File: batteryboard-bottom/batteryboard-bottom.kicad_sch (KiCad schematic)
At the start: 6 parts, among them J1 SLM-110-01-G-S, J2 FTS-105-01-L-DV-A

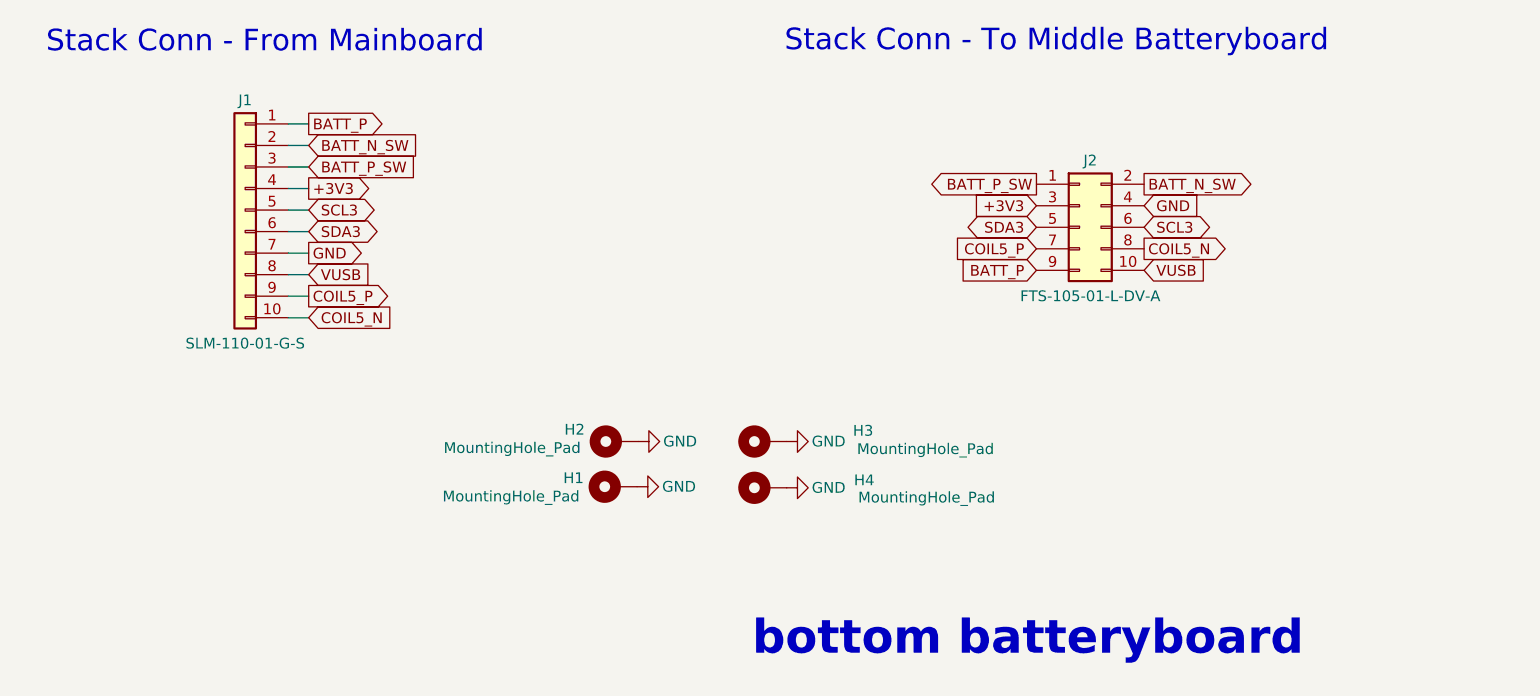
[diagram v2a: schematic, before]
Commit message: Some changes
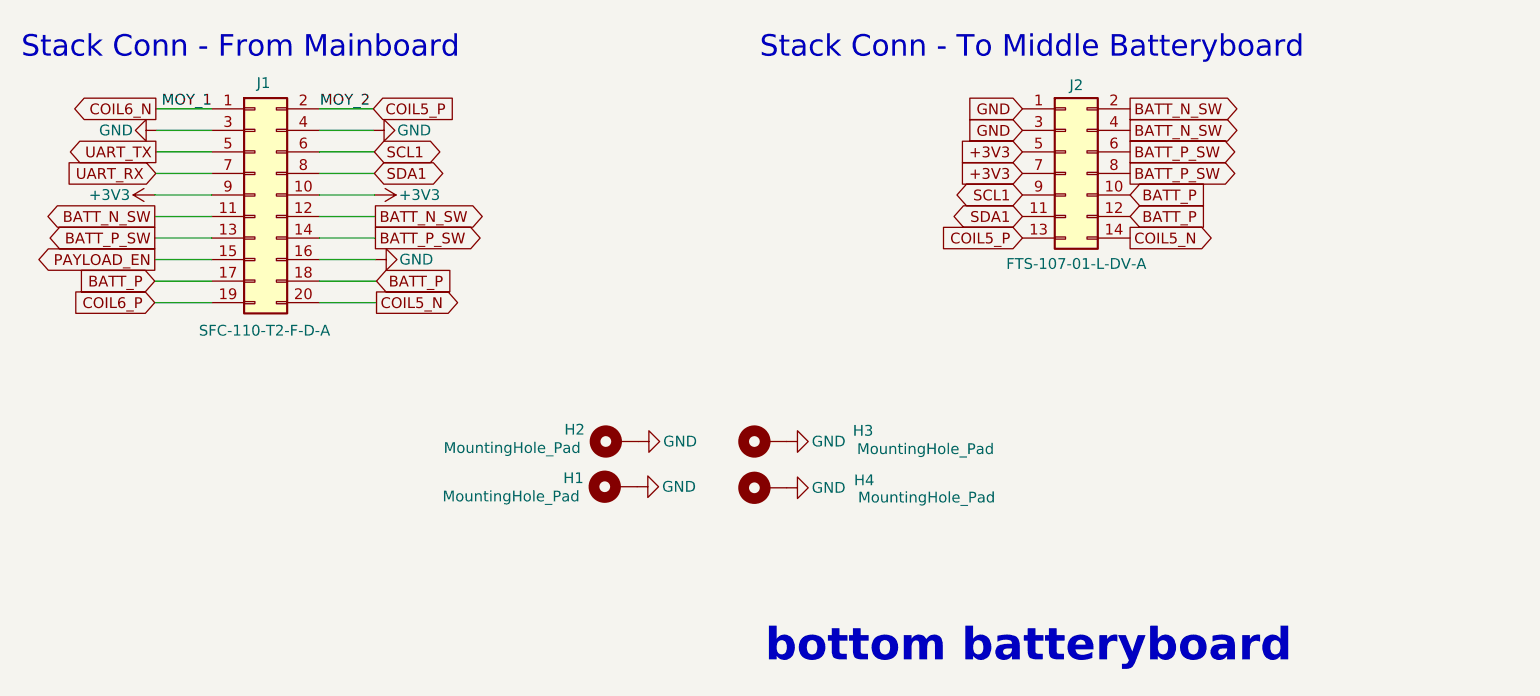
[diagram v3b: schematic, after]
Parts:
- removed J1: SLM-110-01-G-S, batteryboard:SAMTEC_TMS-110-01-G-S, symbol Connector_Generic:Conn_01x10
- removed J2: FTS-105-01-L-DV-A, batteryboard:FTS-105-XX-YY-DV-A, symbol Connector_Generic:Conn_02x05_Odd_Even
- added J1: SFC-110-T2-F-D-A, mainboard:SAMTEC_SFC-110-T2-F-D-A-TR, symbol Connector_Generic:Conn_02x10_Odd_Even
- added J2: FTS-107-01-L-DV-A, batteryboard:SAMTEC-FTS-107-01-X-DV-A, symbol Connector_Generic:Conn_02x07_Odd_Even
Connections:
- net +3V3: now also J1.10 (Pin_10), J1.9 (Pin_9), J2.5 (Pin_5), J2.7 (Pin_7)
- net BATT_N_SW: now also J1.11 (Pin_11), J1.12 (Pin_12), J2.2 (Pin_2), J2.4 (Pin_4)
- net BATT_P: now also J1.17 (Pin_17), J1.18 (Pin_18), J2.10 (Pin_10), J2.12 (Pin_12)
- net BATT_P_SW: now also J1.13 (Pin_13), J1.14 (Pin_14), J2.6 (Pin_6), J2.8 (Pin_8)
- net COIL5_N: now also J1.20 (Pin_20), J2.14 (Pin_14)
- net COIL5_P: now also J1.2 (Pin_2), J2.13 (Pin_13)
- net GND: now also J1.16 (Pin_16), J1.3 (Pin_3), J1.4 (Pin_4), J2.1 (Pin_1), J2.3 (Pin_3)
- new net COIL6_N: J1.1 (Pin_1)
- new net COIL6_P: J1.19 (Pin_19)
- new net PAYLOAD_EN: J1.15 (Pin_15)
- new net SCL1: J1.6 (Pin_6), J2.9 (Pin_9)
- new net SDA1: J1.8 (Pin_8), J2.11 (Pin_11)
- new net UART_RX: J1.7 (Pin_7)
- new net UART_TX: J1.5 (Pin_5)
